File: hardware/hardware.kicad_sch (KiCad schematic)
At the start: 20 parts, among them J1 USB_B_Micro, J3 Conn_02x05_Odd_Even, U1 HY931147C, U28 CH32V307RCT6, U3 LM1117-3.3, U4 CH340C, Y1 Crystal_GND24

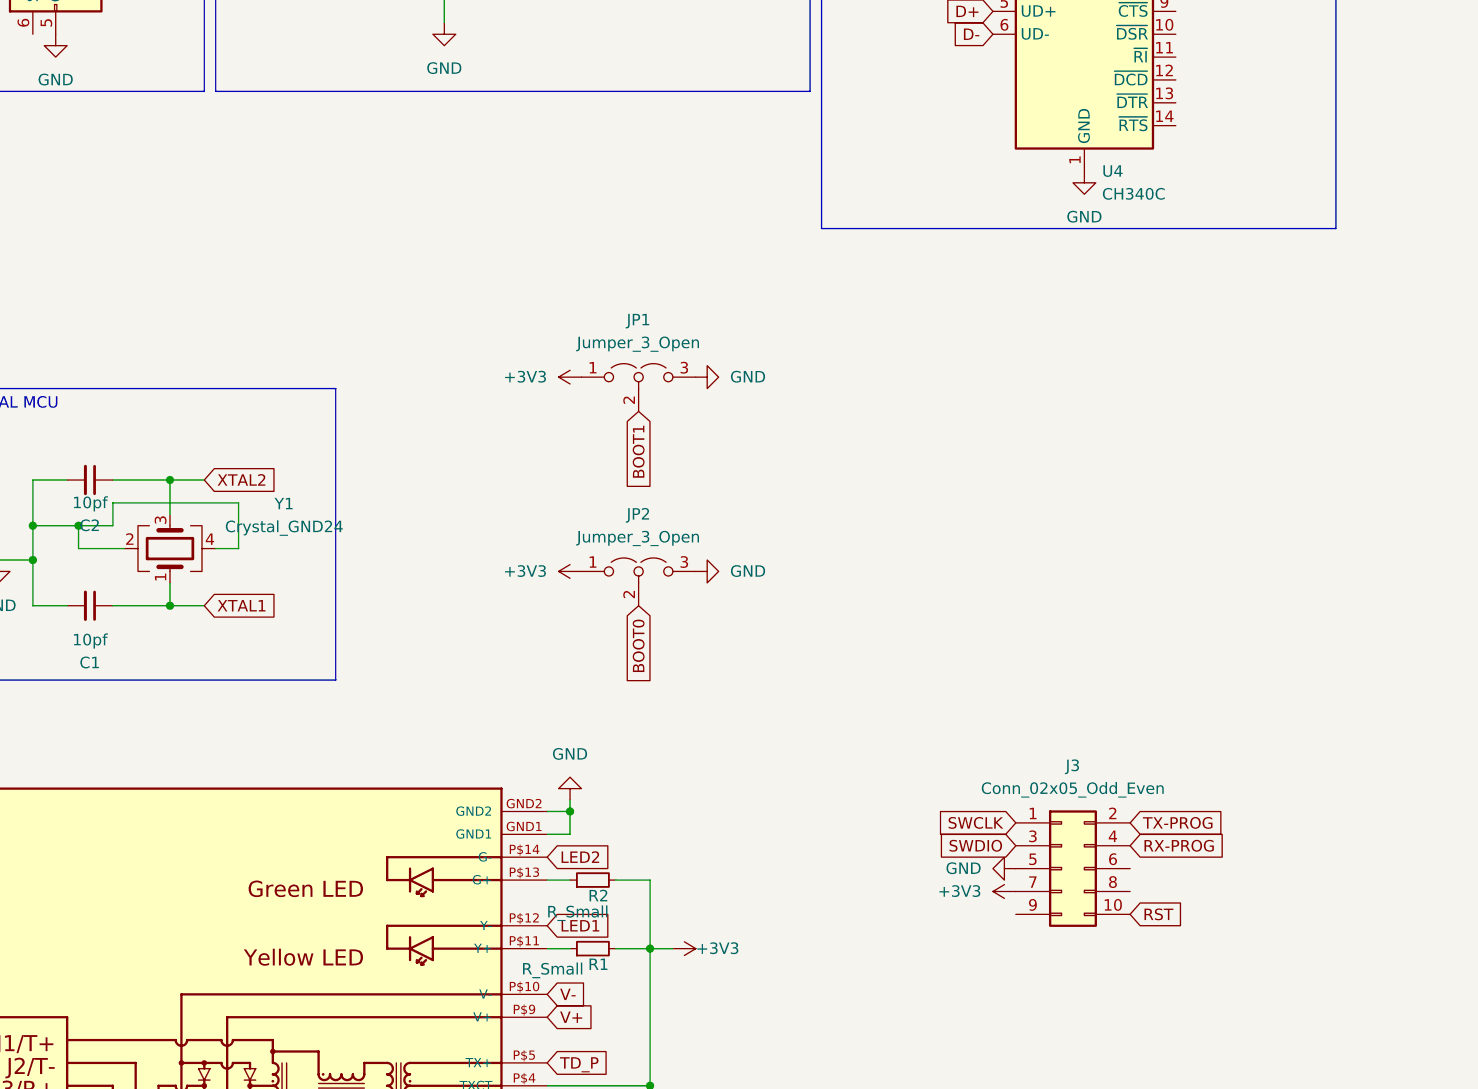
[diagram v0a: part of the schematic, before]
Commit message: wiring pcb
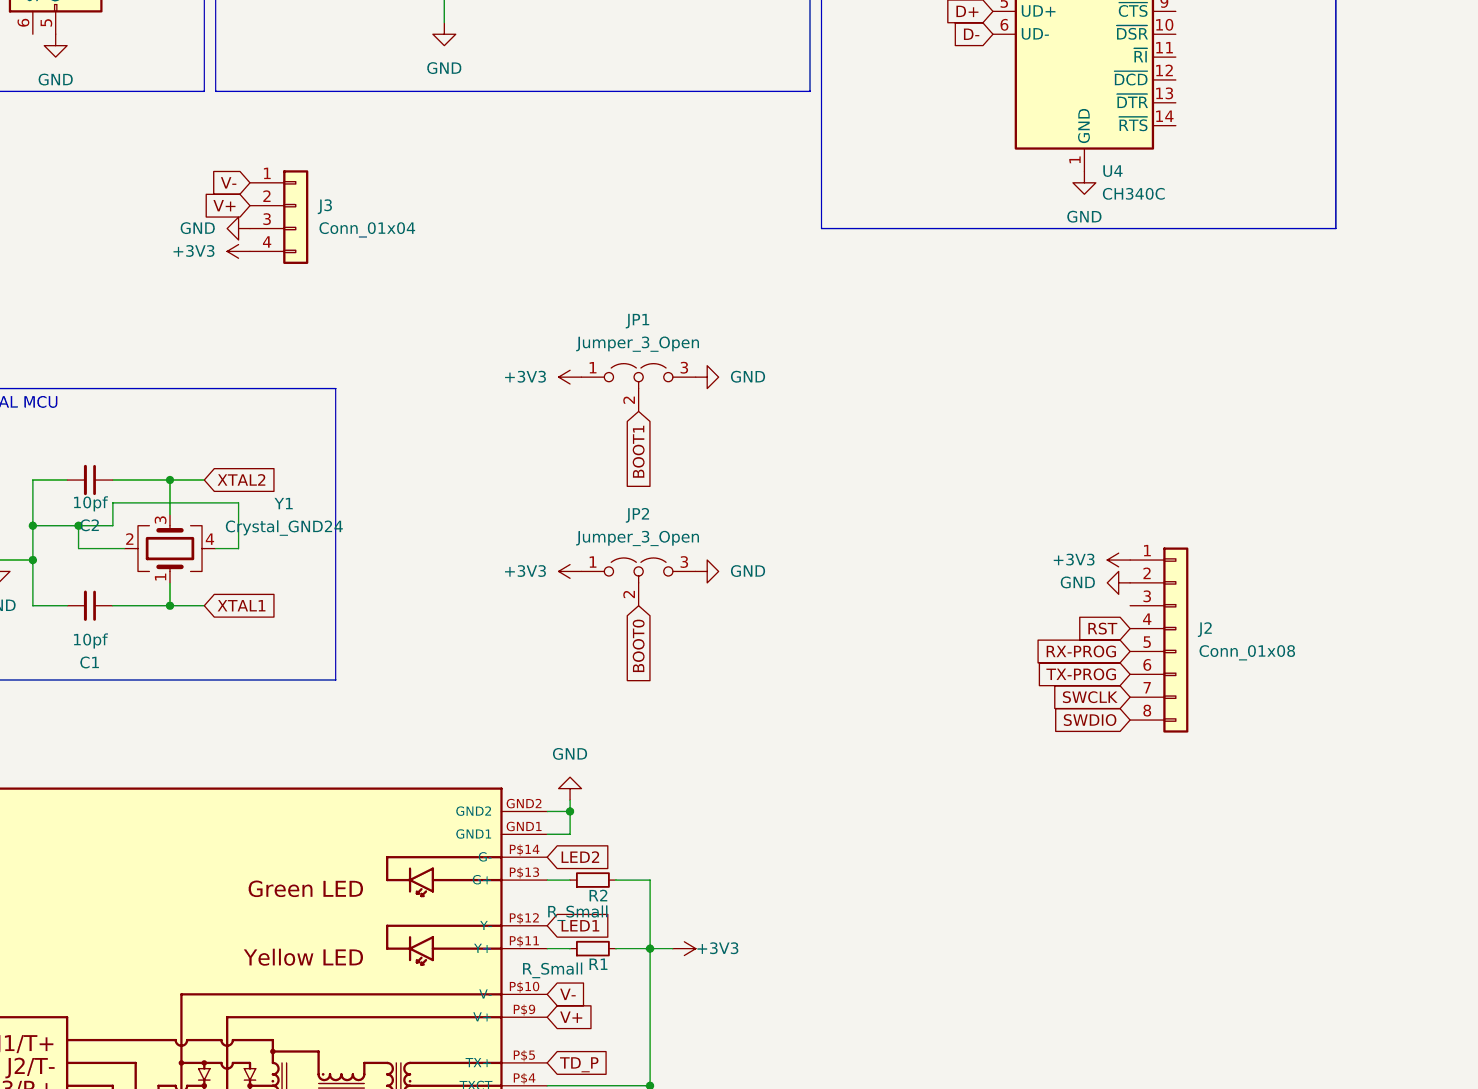
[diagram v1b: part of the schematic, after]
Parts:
- removed J3: Conn_02x05_Odd_Even, Connector_JST:JST_SH_BM10B-SRSS-TB_1x10-1MP_P1.00mm_Vertical, symbol Connector_Generic:Conn_02x05_Odd_Even
- added J2: Conn_01x08, Connector_JST:JST_SH_BM08B-SRSS-TB_1x08-1MP_P1.00mm_Vertical, symbol Connector_Generic:Conn_01x08
- added J3: Conn_01x04, Connector_PinHeader_2.54mm:PinHeader_1x04_P2.54mm_Vertical, symbol Connector_Generic:Conn_01x04
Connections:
- net +3V3: now also J2.1 (Pin_1), J3.4 (Pin_4)
- net GND: now also J2.2 (Pin_2), J3.3 (Pin_3)
- net RST: now also J2.4 (Pin_4)
- net RX-PROG: now also J2.5 (Pin_5)
- net SWCLK: now also J2.7 (Pin_7)
- net SWDIO: now also J2.8 (Pin_8)
- net TX-PROG: now also J2.6 (Pin_6)
- net V+: now also J3.2 (Pin_2)
- net V-: now also J3.1 (Pin_1)
